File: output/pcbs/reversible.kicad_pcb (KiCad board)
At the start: 2 copper layers, 149.1 x 121.9 mm, 72 parts

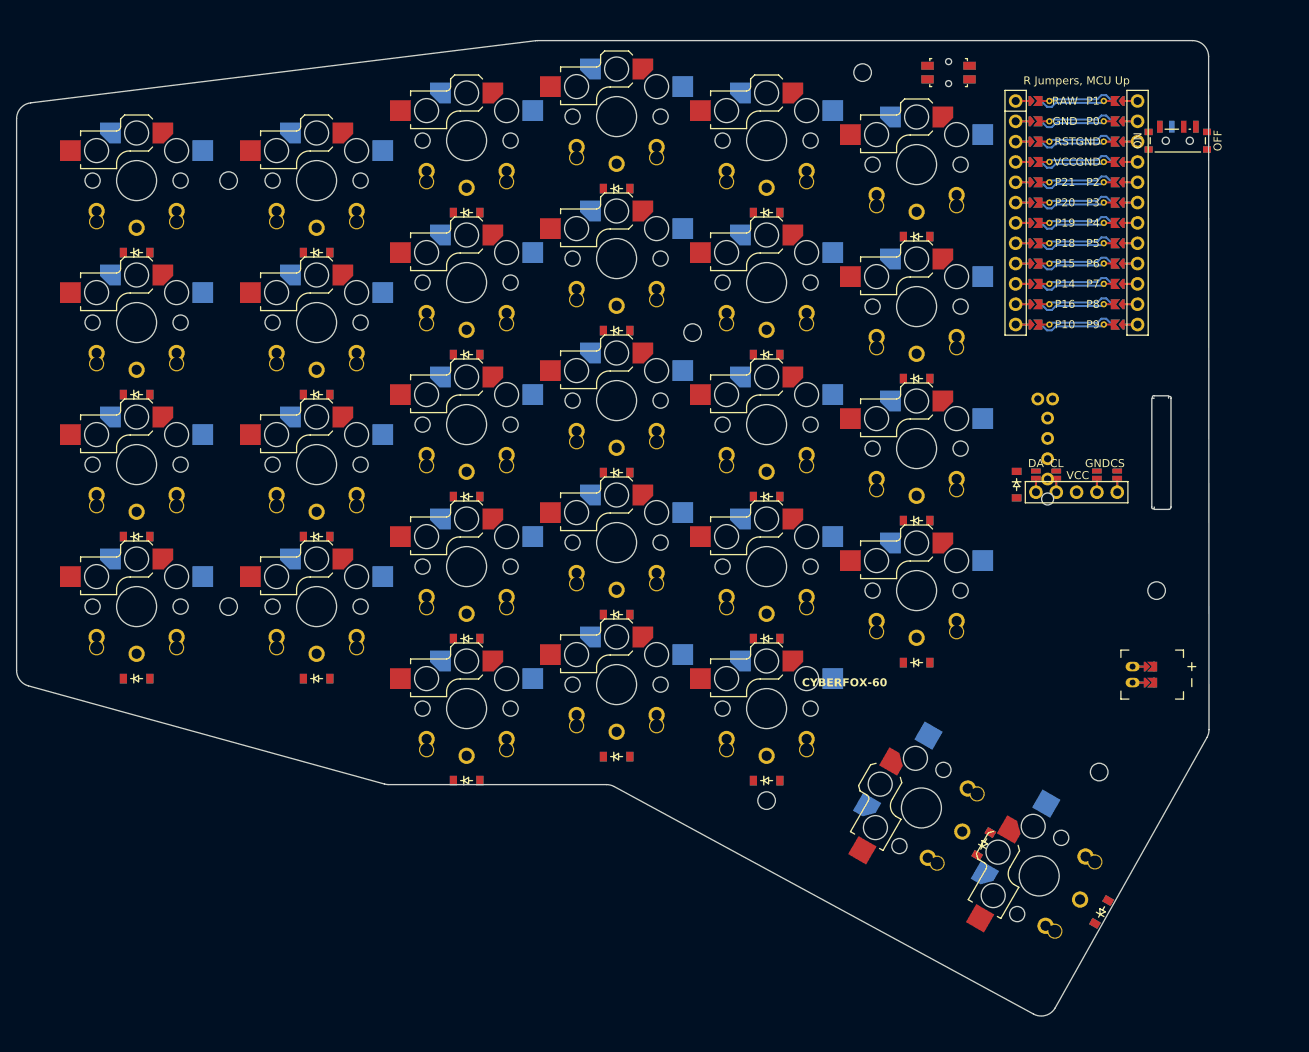
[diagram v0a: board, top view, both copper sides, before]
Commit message: More overhaul. TODO: Need to renet the pins.
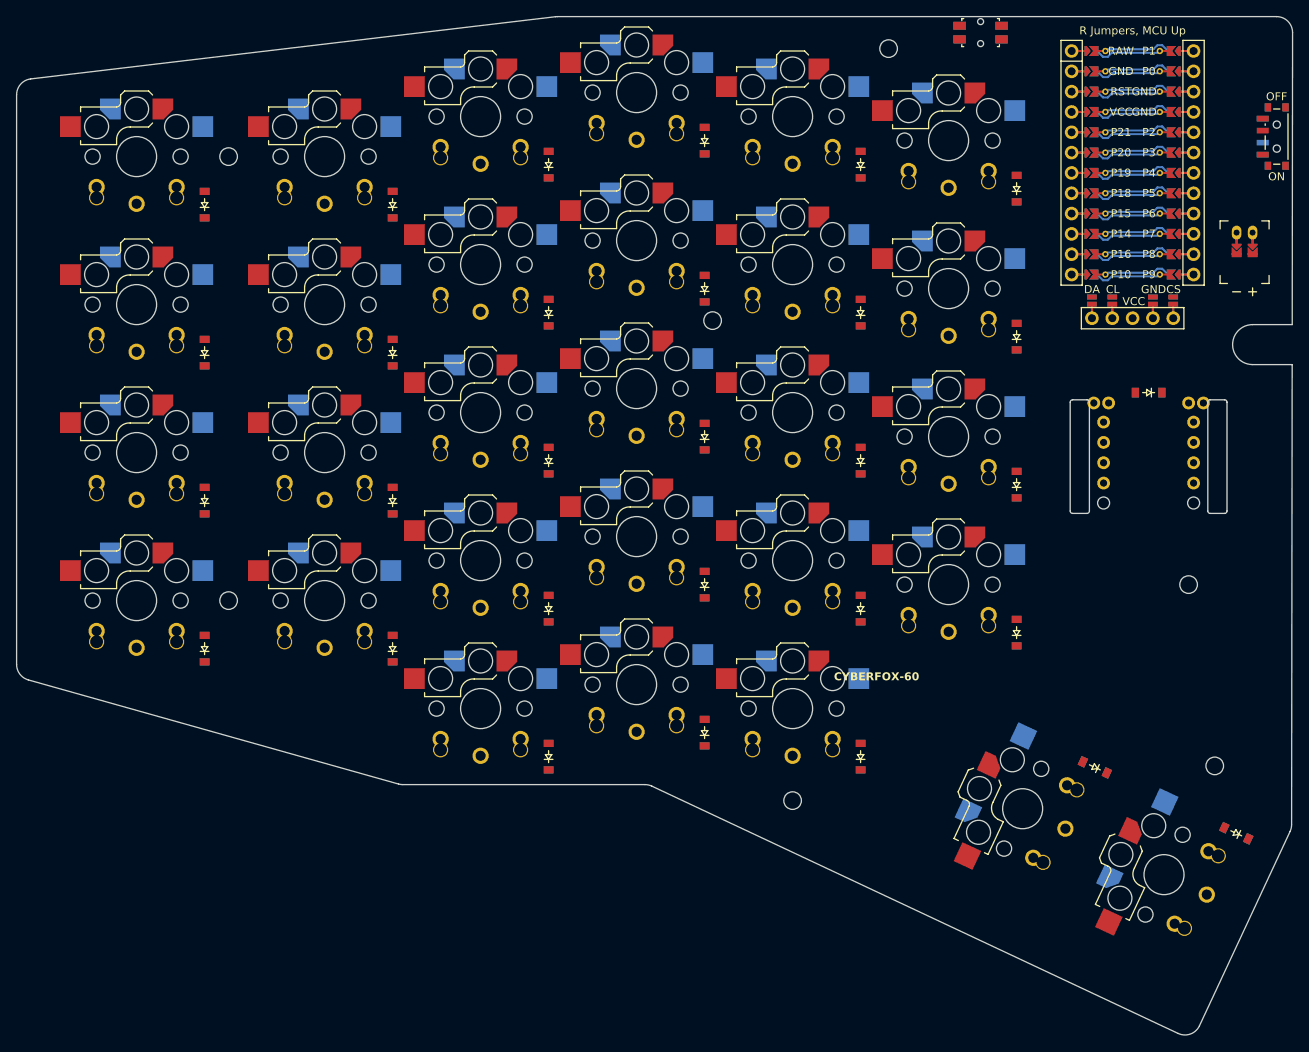
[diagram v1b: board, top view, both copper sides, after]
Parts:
- removed REF**: EVQWGD001, RollerEncoder_Panasonic_EVQWGD001
- added ?: EVQWGD001, RollerEncoder_Panasonic_EVQWGD001, F.Cu at (166.5, 73.0)
- moved JST1 57.0 mm to (178.5, 45.5), turned to 0 degrees
- moved DISP1 22.8 mm to (164.5, 39.5)
- moved D30 20.1 mm to (166.5, 65.5), turned to 180 degrees
- moved D29 19.5 mm to (177.5, 120.6), turned to 155 degrees
- moved D28 16.9 mm to (159.8, 112.3), turned to 155 degrees
- moved S29 15.6 mm to (168.4, 125.8), turned to 65 degrees
- moved MH1 14.5 mm to (174.8, 112.2), turned to 65 degrees
- moved D27 13.9 mm to (150.0, 40.0), turned to 90 degrees
- moved D26 13.6 mm to (150.0, 58.5), turned to 90 degrees
- moved D25 13.3 mm to (150.0, 77.0), turned to 90 degrees
- moved D23 13.2 mm to (130.5, 37.0), turned to 90 degrees
- moved D24 13.1 mm to (150.0, 95.5), turned to 90 degrees
- moved D22 12.9 mm to (130.5, 55.5), turned to 90 degrees
- moved S28 12.7 mm to (150.8, 117.5), turned to 65 degrees
- moved D21 12.6 mm to (130.5, 74.0), turned to 90 degrees
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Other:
- board size 149.1 x 121.9 mm -> 159.5 x 127.3 mm
